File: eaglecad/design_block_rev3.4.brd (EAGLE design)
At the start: 160 x 100 mm, 69 parts, among them Q1 MOSFET-PCH-SOT23-6, Q2 MOSFET-PCH-SOT23-6, Q3 PMV45EN, Q4 PMV45EN, Q5 DMP2240UDM, U1 MAX4211FETE, U2 MAX7310ATE, U3 MIC842LYC5, U4 MIC842LYC5

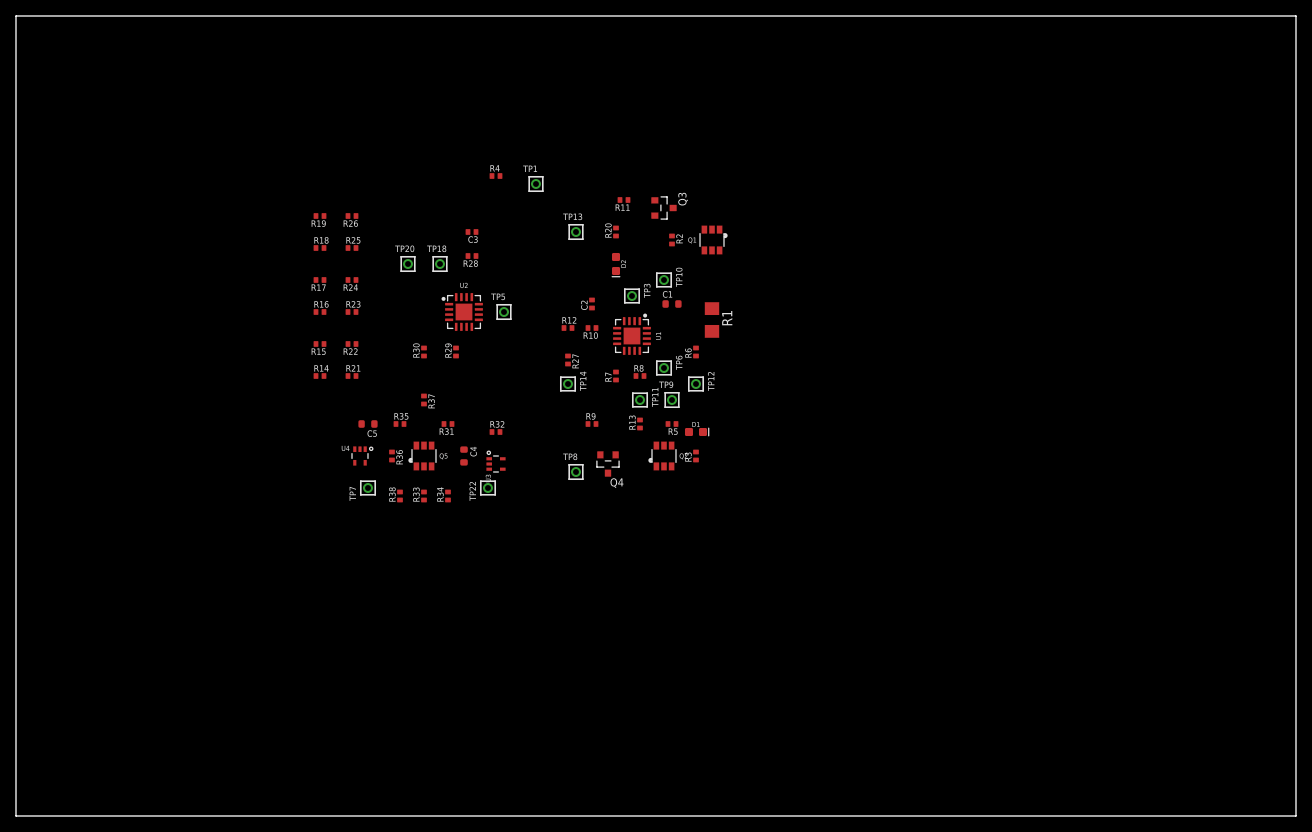
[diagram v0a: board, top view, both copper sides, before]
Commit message: power domain updates
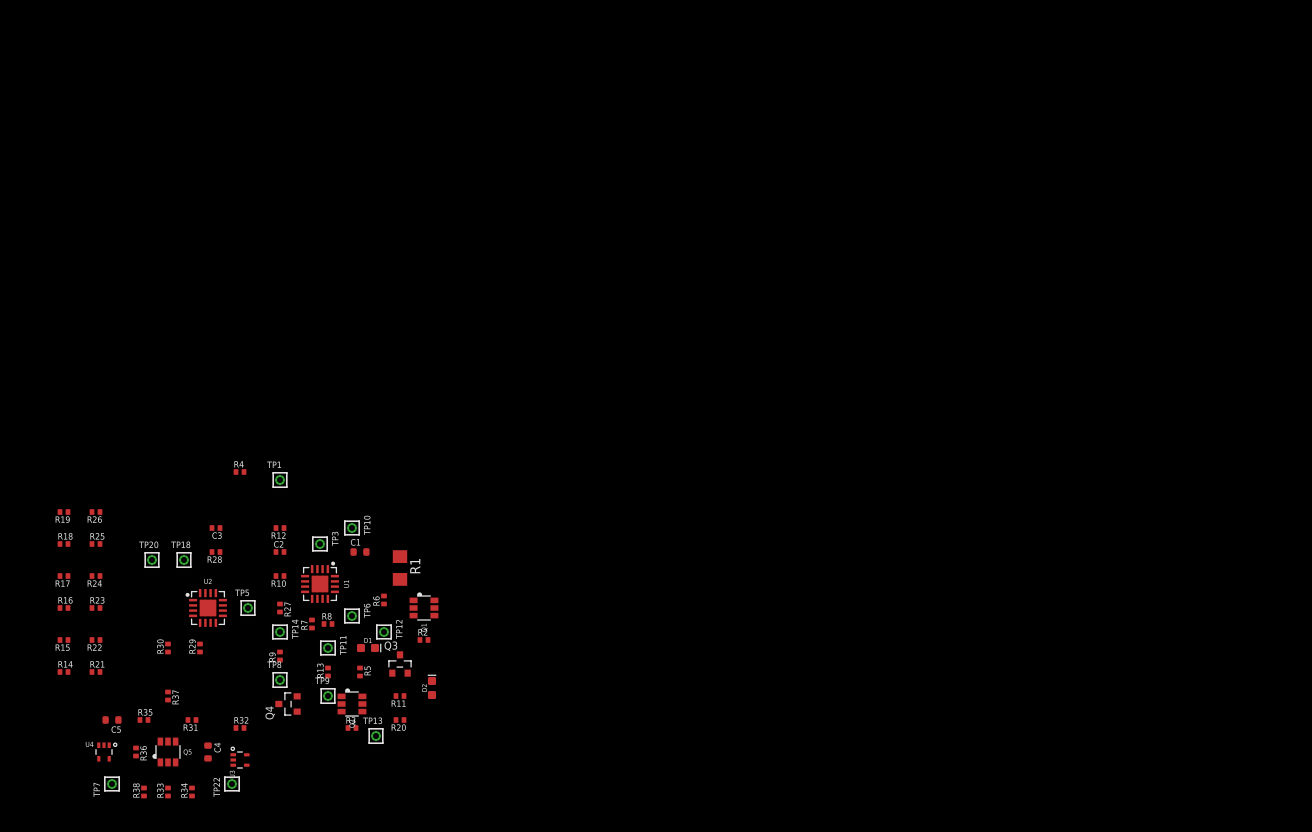
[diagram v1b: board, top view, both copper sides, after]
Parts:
- moved R11 68.0 mm to (48.0, 15.0)
- moved TP13 67.8 mm to (45.0, 10.0)
- moved R20 66.7 mm to (48.0, 12.0), turned to 180 degrees
- moved Q3 65.9 mm to (48.0, 19.0), turned to 0 degrees
- moved R2 58.8 mm to (51.0, 22.0), turned to 0 degrees
- moved Q1 58.4 mm to (51.0, 26.0), turned to 270 degrees
- moved D2 57.8 mm to (52.0, 16.0), turned to 90 degrees
- moved TP9 56.7 mm to (39.0, 15.0)
- moved R3 54.8 mm to (42.0, 11.0), turned to 0 degrees
- moved Q4 50.0 mm to (34.0, 14.0), turned to 90 degrees
- moved C1 49.8 mm to (43.0, 33.0)
- moved C2 49.8 mm to (33.0, 33.0), turned to 0 degrees
- moved Q2 49.8 mm to (42.0, 14.0), turned to 270 degrees
- moved R1 49.8 mm to (48.0, 31.0)
- moved R10 49.8 mm to (33.0, 30.0)
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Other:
- board outline removed
